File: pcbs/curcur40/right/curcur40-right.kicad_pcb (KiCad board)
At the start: 2 copper layers, 124.3 x 91.8 mm, 81 parts

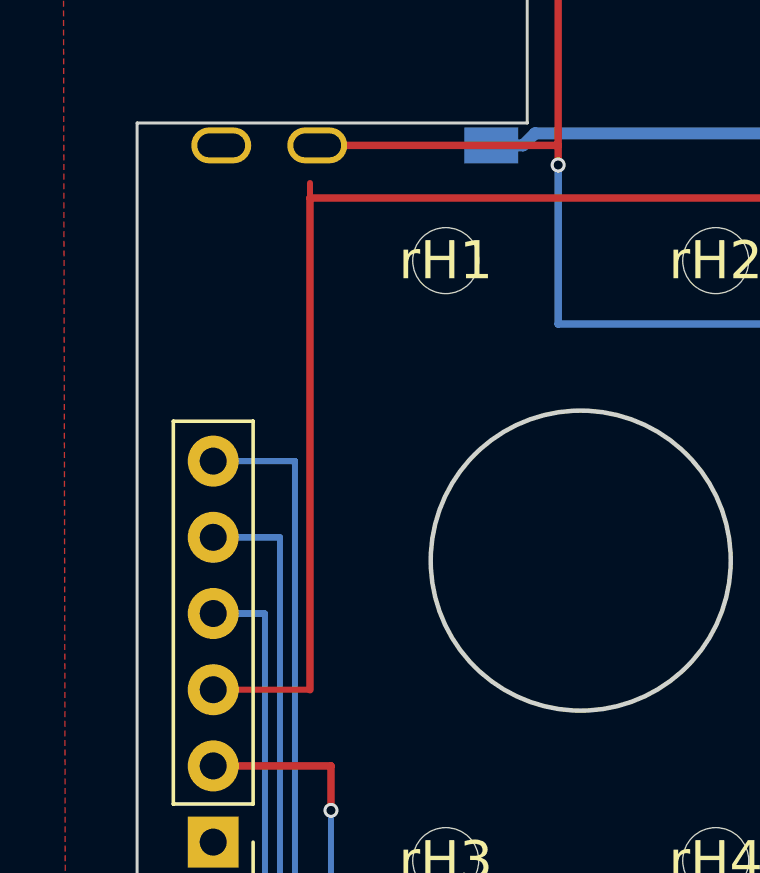
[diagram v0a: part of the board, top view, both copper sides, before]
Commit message: fix
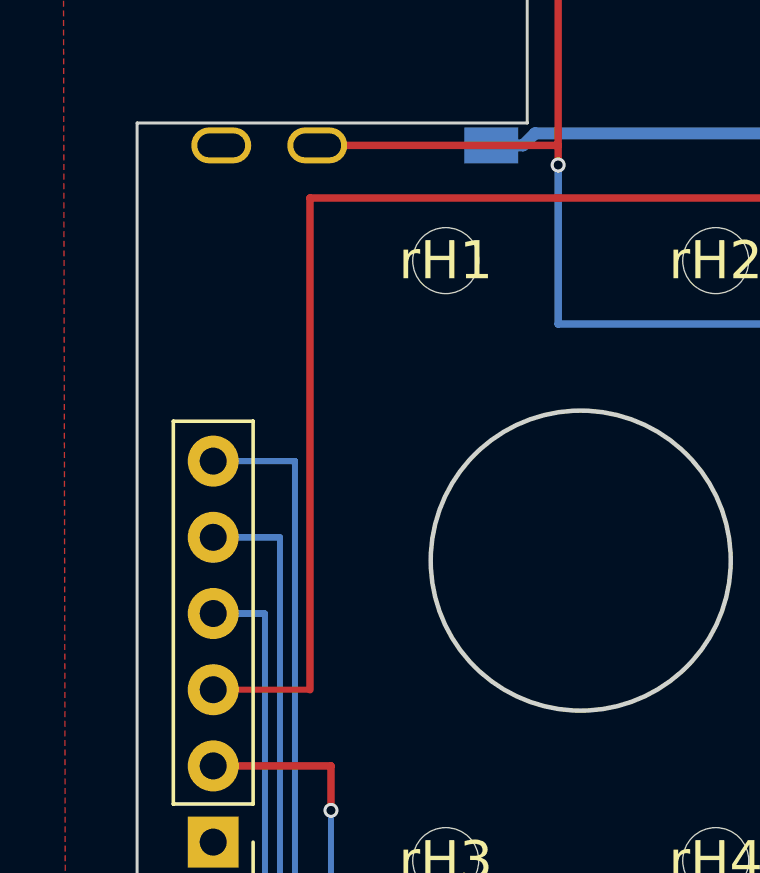
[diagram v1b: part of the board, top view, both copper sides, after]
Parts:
- rU4: footprint Package_SO:SOIC-8_5.23x5.23mm_P1.27mm -> Package_SO:SOIC-8_5.3x5.3mm_P1.27mm
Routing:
- net /NCS: track 170.5 -> 153.6 mm
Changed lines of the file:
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@@
 		)
 	)
-	(footprint "Package_SO:SOIC-8_5.23x5.23mm_P1.27mm"
+	(footprint "Package_SO:SOIC-8_5.3x5.3mm_P1.27mm"
 		(layer "B.Cu")
 		(at 63.1375 13.78625 180)
@@
 		(layer "F.Cu")
 		(net "/NCS")
-	)
-	(segment
-		(start 0.5 39.8)
-		(end 0.5 56.691)
-		(width 0.2)
-		(layer "F.Cu")
-		(net "/NCS")
